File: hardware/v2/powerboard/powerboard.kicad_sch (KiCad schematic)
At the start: 28 parts, among them J1 LEG1_PWR, J10 UBEC3, J11 SBEC, J12 LOGIC_5V_OUT, J13 MONITOR, J2 LEG2_PWR, J3 LEG3_PWR, J4 LEG4_PWR, J5 LEG5_PWR, J6 LEG6_PWR, J7 BATTERY, J8 UBEC1, J9 UBEC2, SW1 MASTER_SW

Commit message: Update V2 board schematics and footprints
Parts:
- D2, D3, D4, D5: footprint (none) -> LED_SMD:LED_0805_2012Metric
- R1, R2, R3, R4: footprint (none) -> Resistor_SMD:R_0805_2012Metric
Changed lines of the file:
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@@
 			)
 		)
-		(property "Footprint" ""
+		(property "Footprint" "Resistor_SMD:R_0805_2012Metric"
 			(at 60 75 0)
 			(effects
@@
 			)
 		)
-		(property "Footprint" ""
+		(property "Footprint" "LED_SMD:LED_0805_2012Metric"
 			(at 60 88 0)
 			(effects
@@
 			)
 		)
-		(property "Footprint" ""
+		(property "Footprint" "Resistor_SMD:R_0805_2012Metric"
 			(at 100 75 0)
 			(effects
@@
 			)
 		)
-		(property "Footprint" ""
+		(property "Footprint" "LED_SMD:LED_0805_2012Metric"
 			(at 100 88 0)
 			(effects
@@
 			)
 		)
-		(property "Footprint" ""
+		(property "Footprint" "Resistor_SMD:R_0805_2012Metric"
 			(at 140 75 0)
 			(effects
@@
 			)
 		)
-		(property "Footprint" ""
+		(property "Footprint" "LED_SMD:LED_0805_2012Metric"
 			(at 140 88 0)
 			(effects
@@
 			)
 		)
-		(property "Footprint" ""
+		(property "Footprint" "Resistor_SMD:R_0805_2012Metric"
 			(at 180 75 0)
 			(effects
@@
 			)
 		)
-		(property "Footprint" ""
+		(property "Footprint" "LED_SMD:LED_0805_2012Metric"
 			(at 180 88 0)
 			(effects

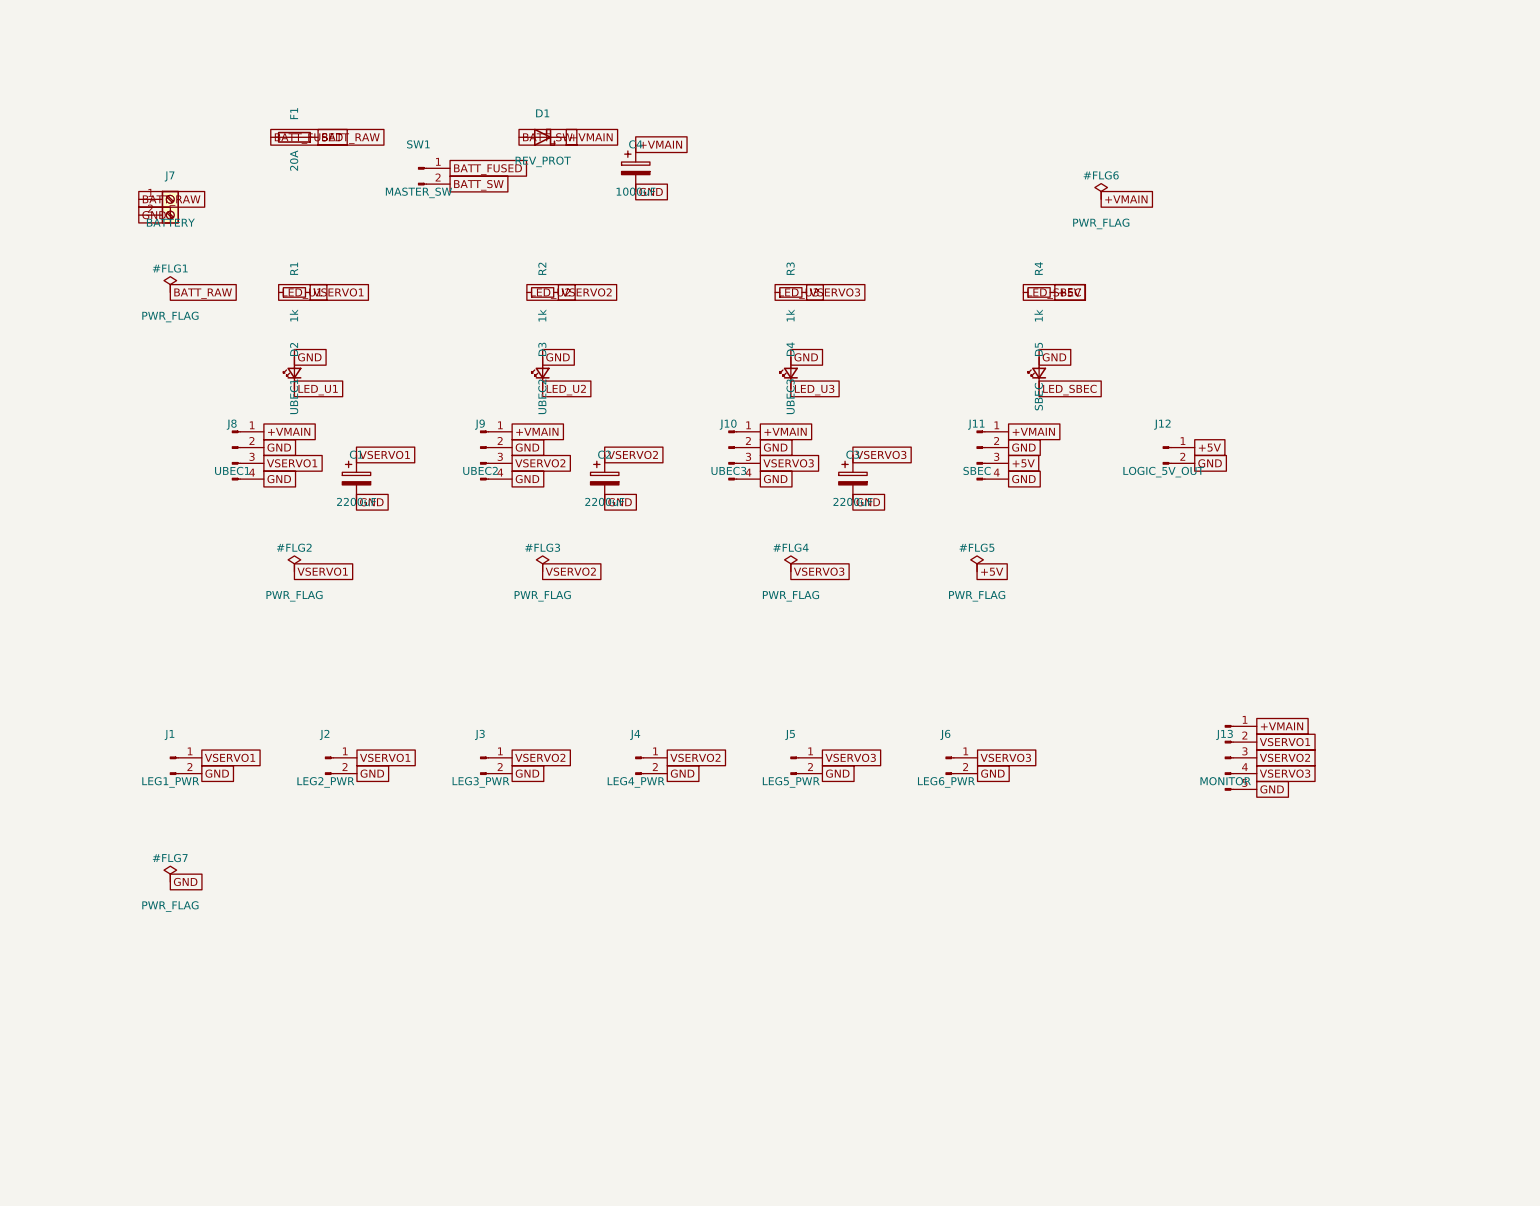
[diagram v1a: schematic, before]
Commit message: powerboard changes
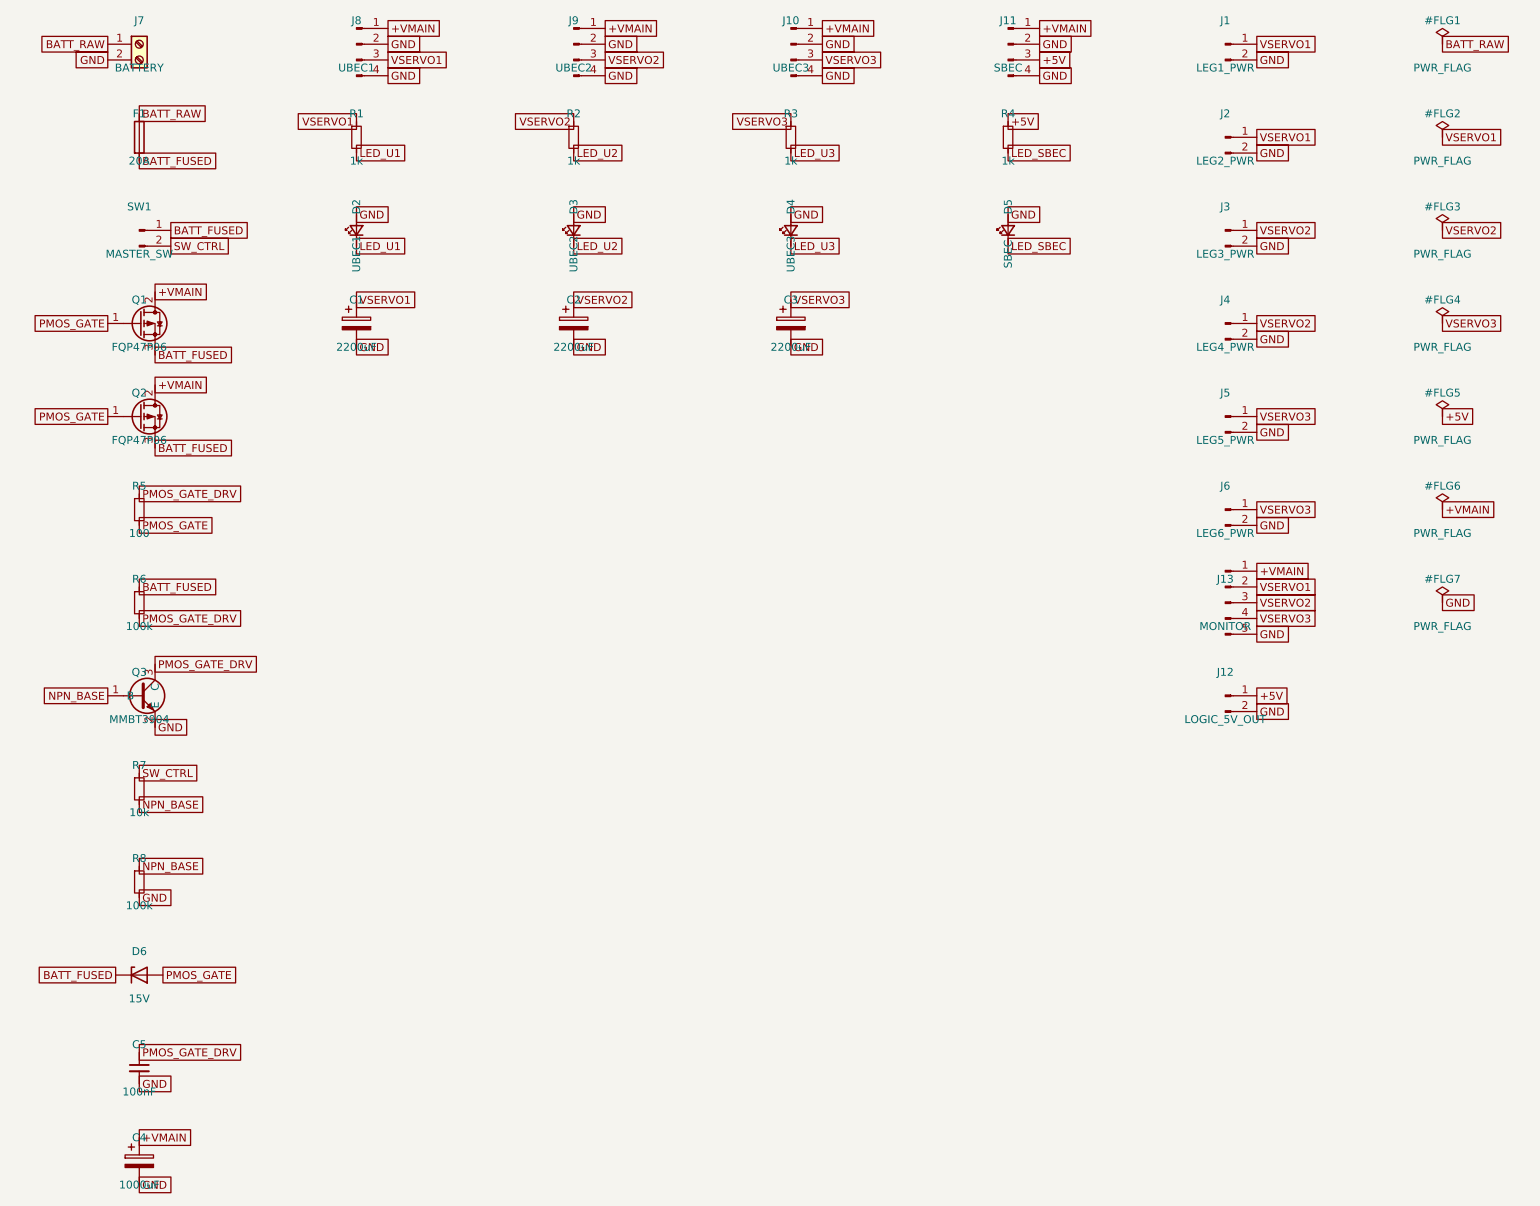
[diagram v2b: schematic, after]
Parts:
- removed D1: REV_PROT, symbol Device:D_Schottky
- added C5: 100nF, Capacitor_SMD:C_0805_2012Metric, symbol Device:C_Small
- added D6: 15V, Diode_SMD:D_0805_2012Metric, symbol Device:D_Zener
- added Q1, Q2: FQP47P06, Package_TO_SOT_THT:TO-220-3_Vertical, symbol Transistor_FET:Q_PMOS_GDS
- added Q3: MMBT3904, Package_TO_SOT_SMD:SOT-23, symbol SymbolsLib:MMBT3904
- added R5: 100, Resistor_SMD:R_0805_2012Metric, symbol Device:R_Small
- added R6, R8: 100k, Resistor_SMD:R_0805_2012Metric, symbol Device:R_Small
- added R7: 10k, Resistor_SMD:R_0805_2012Metric, symbol Device:R_Small
- C1, C2, C3: footprint (none) -> Capacitor_THT:CP_Radial_D13.0mm_P5.00mm
- C4: footprint (none) -> Capacitor_THT:CP_Radial_D8.0mm_P3.80mm
- F1: footprint (none) -> Custom:Fuse Holder Mini
- J1, J2, J3, J4, J5, J6: footprint (none) -> TerminalBlock:TerminalBlock_MaiXu_MX126-5.0-02P_1x02_P5.00mm
- J10, J11, J8, J9: footprint (none) -> Connector_Wire:SolderWire-0.25sqmm_1x04_P4.2mm_D0.65mm_OD1.7mm
- J12: footprint (none) -> Connector_PinHeader_2.54mm:PinHeader_1x02_P2.54mm_Vertical
- J13: footprint (none) -> Connector_PinHeader_2.54mm:PinHeader_1x05_P2.54mm_Vertical
- J7: footprint (none) -> Connector_Wire:SolderWire-1.5sqmm_1x02_P7.8mm_D1.7mm_OD3.9mm
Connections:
- net +5V: now also R4.1; no longer R4.2
- net +VMAIN: now also Q1.2 (D), Q2.2 (D)
- net BATT_FUSED: now also F1.2, D6.1 (K), Q1.3 (S), Q2.3 (S), R6.1; no longer F1.1
- net BATT_RAW: now also F1.1; no longer F1.2
- net GND: now also C5.2, Q3.2 (E), R8.2
- net LED_SBEC: now also R4.2; no longer R4.1
- net LED_U1: now also R1.2; no longer R1.1
- net LED_U2: now also R2.2; no longer R2.1
- net LED_U3: now also R3.2; no longer R3.1
- net VSERVO1: now also R1.1; no longer R1.2
- net VSERVO2: now also R2.1; no longer R2.2
- net VSERVO3: now also R3.1; no longer R3.2
- net BATT_SW renamed SW_CTRL
- net SW_CTRL: now also R7.1
- new net NPN_BASE: Q3.1 (B), R7.2, R8.1
- new net PMOS_GATE: D6.2 (A), Q1.1 (G), Q2.1 (G), R5.2
- new net PMOS_GATE_DRV: C5.1, Q3.3 (C), R5.1, R6.2
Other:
- moved on the sheet: C1, C2, C3, C4, D2, D3, D4, D5, F1, J1, J10, J11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

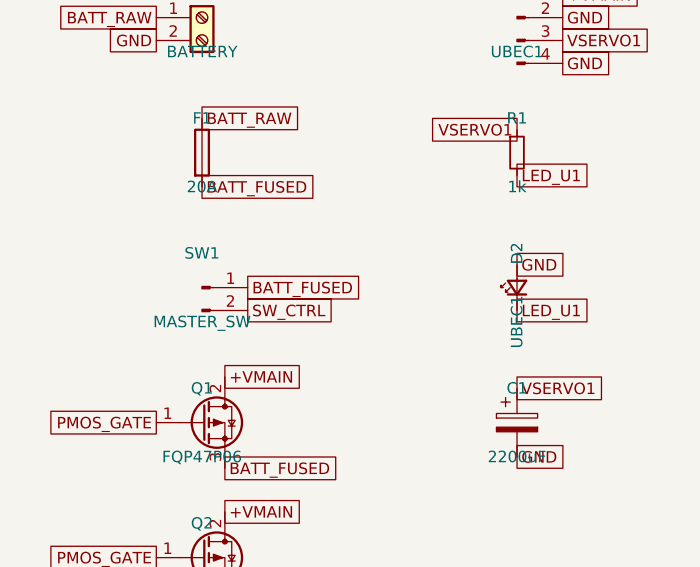
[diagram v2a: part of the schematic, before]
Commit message: powerboard layout
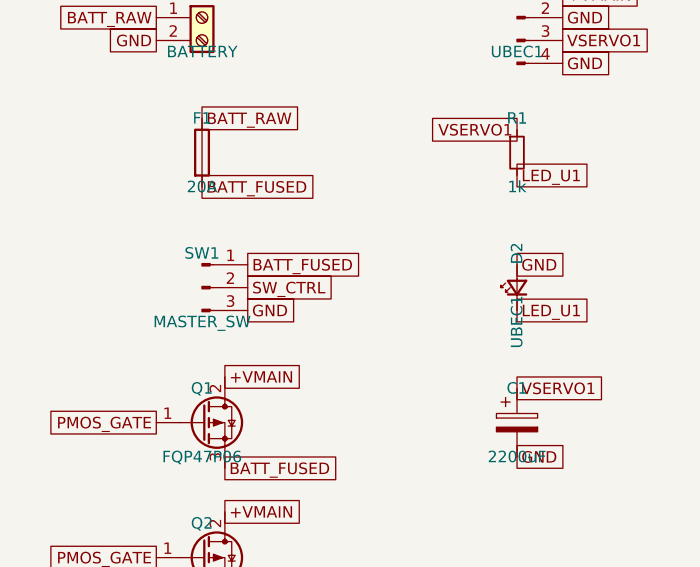
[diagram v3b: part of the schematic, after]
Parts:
- SW1: footprint (none) -> Custom:SW_Slide_SPDT_Straight; symbol Connector:Conn_01x02_Pin -> Connector:Conn_01x03_Pin
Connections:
- net GND: now also SW1.3 (Pin_3)
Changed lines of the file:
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@@
 	)
 	(symbol
-		(lib_id "Connector:Conn_01x02_Pin")
+		(lib_id "Connector:Conn_01x03_Pin")
 		(at 35 65 0)
 		(unit 1)
@@
 			)
 		)
-		(property "Footprint" ""
+		(property "Footprint" "Custom:SW_Slide_SPDT_Straight"
 			(at 35 65 0)
 			(effects
@@
 	(global_label "BATT_FUSED"
 		(shape passive)
-		(at 40.08 65 0)
+		(at 40.08 62.46 0)
+		(fields_autoplaced yes)
+		(effects
+			(font
+				(size 1.27 1.27)
+			)
+			(justify left)
+		)
+	)
+	(global_label "GND"
+		(shape passive)
+		(at 40.08 67.54 0)
 		(fields_autoplaced yes)
 		(effects
@@
 	(global_label "SW_CTRL"
 		(shape passive)
-		(at 40.08 67.54 0)
-		(fields_autoplaced yes)
-		(effects
+		(at 40.08 65 0)
+		(fields_autoplaced yes)
+		(effects
